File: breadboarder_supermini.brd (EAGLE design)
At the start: 70.8 x 34.3 mm, 22 parts, among them IC1 AVR-MEGA8-PPTH, Q1 MOSFET-NCHANNEL2N7000

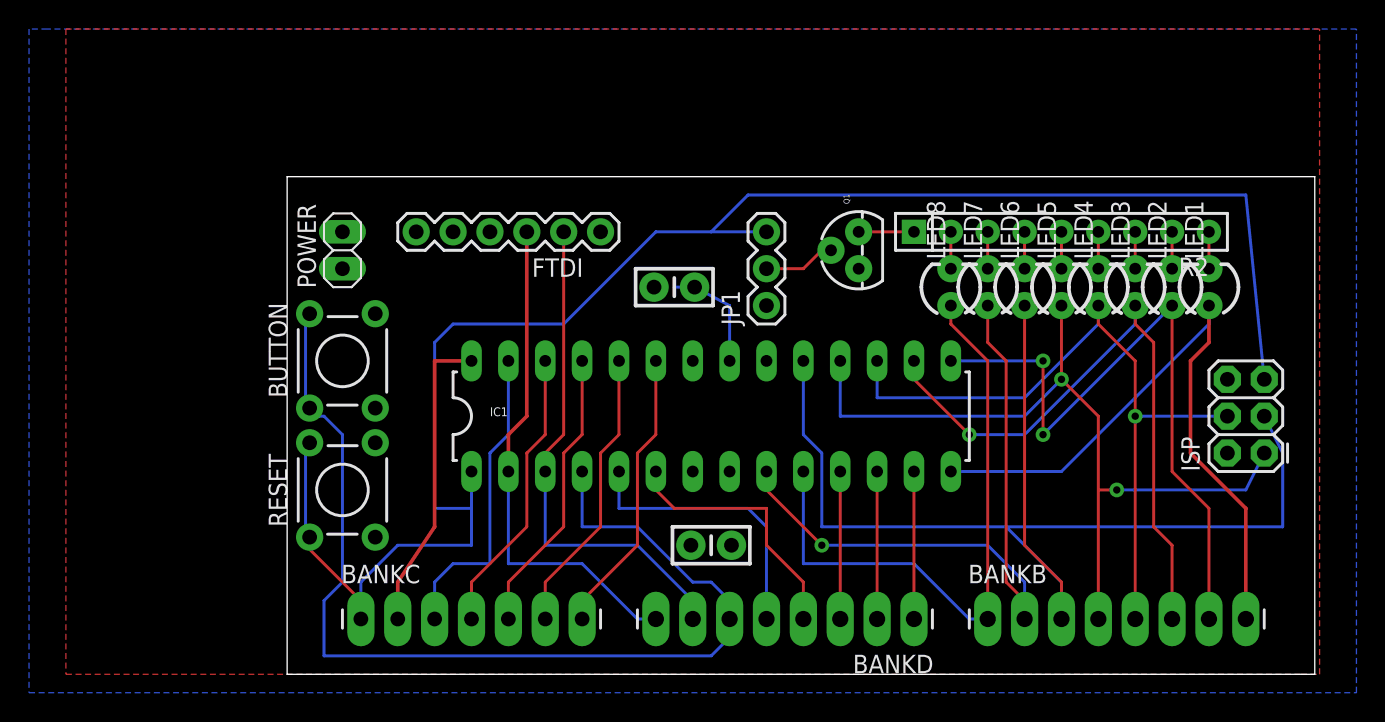
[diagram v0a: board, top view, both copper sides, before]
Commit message: tested version minimal classboard
is it a minimal classboard or a mega breadboarder?
8-LED breakout untested, mostly-symmetric design
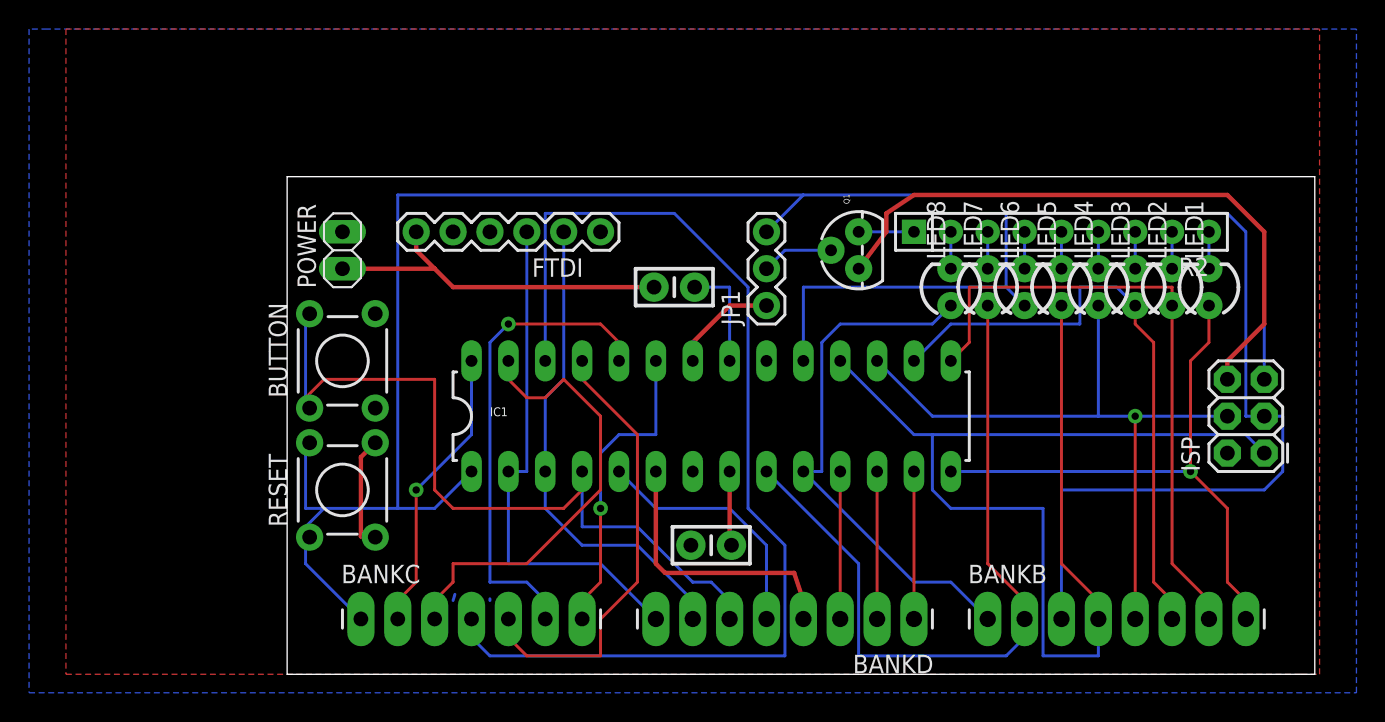
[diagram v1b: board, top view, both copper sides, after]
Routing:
- net GND: track 0.00 -> 89.2 mm
- net PC3: track 19.9 -> 76.1 mm
- net PB4: track 55.7 -> 82.9 mm, vias 2 -> 0
- net PD2: track 73.1 -> 54.2 mm
- net PC1: track 19.9 -> 33.3 mm, vias 0 -> 1
- net PC2: track 19.9 -> 31.1 mm
- net PC4: track 21.4 -> 31.4 mm
- net PB0: track 47.0 -> 40.2 mm, vias 0 -> 1
- net PB7: track 43.3 -> 37.0 mm
- net PB5: track 82.2 -> 86.7 mm
- net PB6: track 46.9 -> 51.2 mm, vias 1 -> 0
- net PB2: track 45.2 -> 42.0 mm, vias 1 -> 0
- net PB1: track 46.6 -> 43.5 mm, vias 2 -> 0
- net PB3: track 50.1 -> 47.3 mm
- net PD3: track 19.6 -> 17.3 mm
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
